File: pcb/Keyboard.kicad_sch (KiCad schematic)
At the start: 63 parts

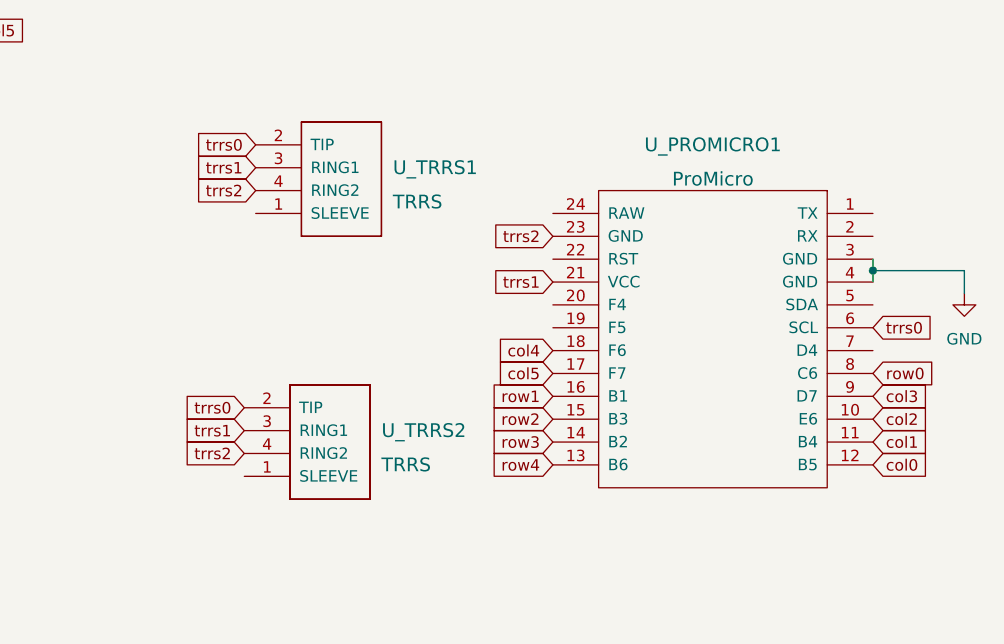
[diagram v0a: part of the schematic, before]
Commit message: wip
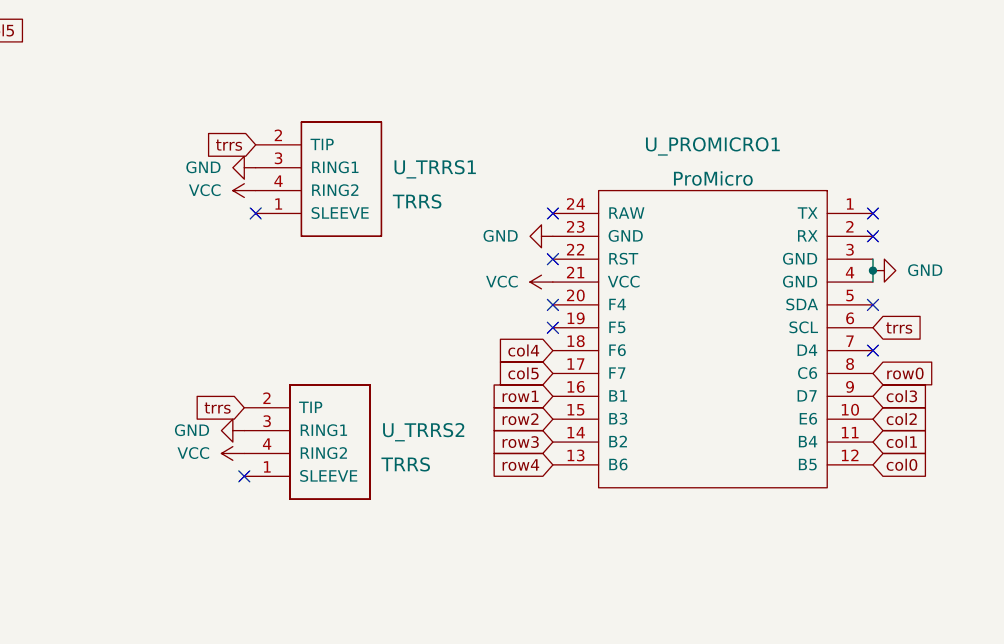
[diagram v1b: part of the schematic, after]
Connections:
- net GND: now also U_PROMICRO1.23 (GND), U_TRRS1.3 (RING1), U_TRRS2.3 (RING1)
- net trrs0 renamed trrs
- removed net trrs1: U_PROMICRO1.21 (VCC), U_TRRS1.3 (RING1), U_TRRS2.3 (RING1)
- net trrs2 renamed VCC
- net VCC: now also U_PROMICRO1.21 (VCC); no longer U_PROMICRO1.23 (GND)
- no-connect marks 0 -> 10

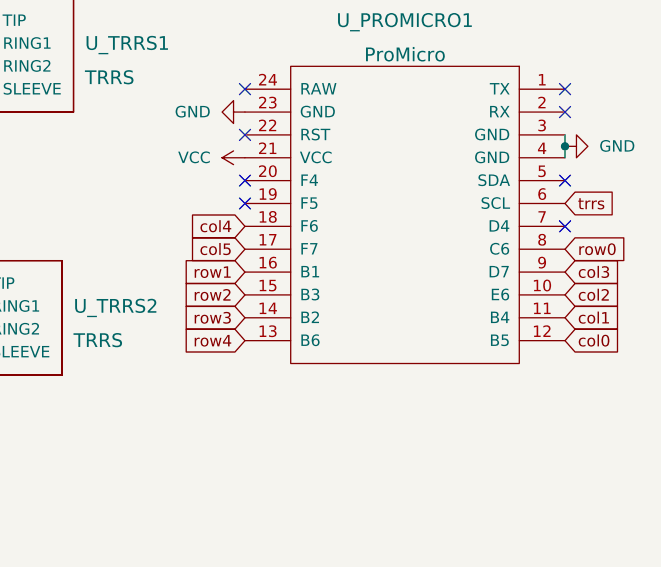
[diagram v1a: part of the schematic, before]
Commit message: wip
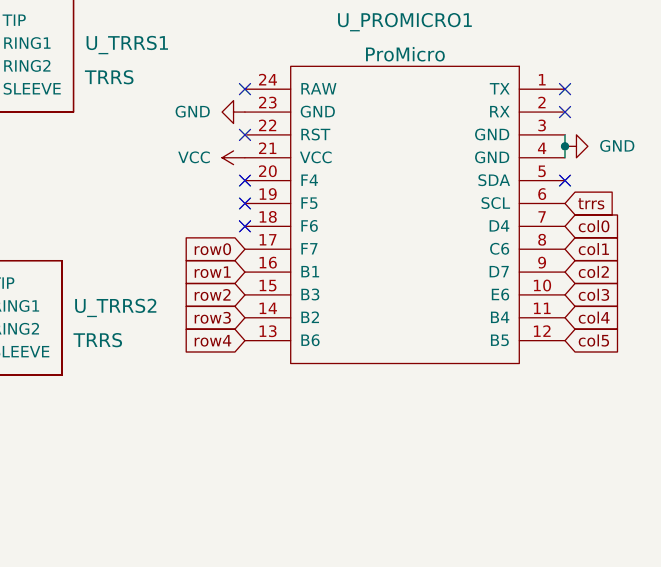
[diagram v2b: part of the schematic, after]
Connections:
- net col0: now also U_PROMICRO1.7 (D4); no longer U_PROMICRO1.12 (B5)
- net col1: now also U_PROMICRO1.8 (C6); no longer U_PROMICRO1.11 (B4)
- net col2: now also U_PROMICRO1.9 (D7); no longer U_PROMICRO1.10 (E6)
- net col3: now also U_PROMICRO1.10 (E6); no longer U_PROMICRO1.9 (D7)
- net col4: now also U_PROMICRO1.11 (B4); no longer U_PROMICRO1.18 (F6)
- net col5: now also U_PROMICRO1.12 (B5); no longer U_PROMICRO1.17 (F7)
- net row0: now also U_PROMICRO1.17 (F7); no longer U_PROMICRO1.8 (C6)
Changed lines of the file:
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@@
   (no_connect (at 262.89 45.72))
   (no_connect (at 262.89 43.18))
-  (no_connect (at 262.89 58.42))
+  (no_connect (at 227.33 58.42))
   (no_connect (at 193.04 72.39))
   (no_connect (at 194.31 43.18))
@@
     (stroke (width 0) (type default) (color 0 0 0 0))
   )
-  (global_label "col5" (shape input) (at 227.33 60.96 180) (fields_autoplaced)
-    (effects (font (size 1.27 1.27)) (justify right))
-    (property "Intersheet References" "${INTERSHEET_REFS}" (id 0) (at 220.8045 60.8806 0)
-      (effects (font (size 1.27 1.27)) (justify right) hide)
-    )
-  )
-  (global_label "col3" (shape input) (at 262.89 63.5 0) (fields_autoplaced)
+  (global_label "col5" (shape input) (at 262.89 71.12 0) (fields_autoplaced)
+    (effects (font (size 1.27 1.27)) (justify left))
+    (property "Intersheet References" "${INTERSHEET_REFS}" (id 0) (at 269.4155 71.0406 0)
+      (effects (font (size 1.27 1.27)) (justify left) hide)
+    )
+  )
+  (global_label "col3" (shape input) (at 262.89 66.04 0) (fields_autoplaced)
+    (effects (font (size 1.27 1.27)) (justify left))
+    (property "Intersheet References" "${INTERSHEET_REFS}" (id 0) (at 269.4155 65.9606 0)
+      (effects (font (size 1.27 1.27)) (justify left) hide)
+    )
+  )
+  (global_label "row4" (shape input) (at 227.33 71.12 180) (fields_autoplaced)
+    (effects (font (size 1.27 1.27)) (justify right))
+    (property "Intersheet References" "${INTERSHEET_REFS}" (id 0) (at 220.4417 71.0406 0)
+      (effects (font (size 1.27 1.27)) (justify right) hide)
+    )
+  )
+  (global_label "trrs" (shape input) (at 194.31 35.56 180) (fields_autoplaced)
+    (effects (font (size 1.27 1.27)) (justify right))
+    (property "Intersheet References" "${INTERSHEET_REFS}" (id 0) (at 188.5707 35.4806 0)
+      (effects (font (size 1.27 1.27)) (justify right) hide)
+    )
+  )
+  (global_label "col4" (shape input) (at 138.43 22.86 0) (fields_autoplaced)
+    (effects (font (size 1.27 1.27)) (justify left))
+    (property "Intersheet References" "${INTERSHEET_REFS}" (id 0) (at 144.9555 22.7806 0)
+      (effects (font (size 1.27 1.27)) (justify left) hide)
+    )
+  )
+  (global_label "row2" (shape input) (at 227.33 66.04 180) (fields_autoplaced)
+    (effects (font (size 1.27 1.27)) (justify right))
+    (property "Intersheet References" "${INTERSHEET_REFS}" (id 0) (at 220.4417 65.9606 0)
+      (effects (font (size 1.27 1.27)) (justify right) hide)
+    )
+  )
+  (global_label "trrs" (shape input) (at 262.89 55.88 0) (fields_autoplaced)
+    (effects (font (size 1.27 1.27)) (justify left))
+    (property "Intersheet References" "${INTERSHEET_REFS}" (id 0) (at 268.6293 55.8006 0)
+      (effects (font (size 1.27 1.27)) (justify left) hide)
+    )
+  )
+  (global_label "col1" (shape input) (at 66.04 22.86 0) (fields_autoplaced)
+    (effects (font (size 1.27 1.27)) (justify left))
+    (property "Intersheet References" "${INTERSHEET_REFS}" (id 0) (at 72.5655 22.7806 0)
+      (effects (font (size 1.27 1.27)) (justify left) hide)
+    )
+  )
+  (global_label "col2" (shape input) (at 262.89 63.5 0) (fields_autoplaced)
     (effects (font (size 1.27 1.27)) (justify left))
     (property "Intersheet References" "${INTERSHEET_REFS}" (id 0) (at 269.4155 63.4206 0)
@@
     )
   )
-  (global_label "row4" (shape input) (at 227.33 71.12 180) (fields_autoplaced)
-    (effects (font (size 1.27 1.27)) (justify right))
-    (property "Intersheet References" "${INTERSHEET_REFS}" (id 0) (at 220.4417 71.0406 0)
-      (effects (font (size 1.27 1.27)) (justify right) hide)
-    )
-  )
-  (global_label "trrs" (shape input) (at 194.31 35.56 180) (fields_autoplaced)
-    (effects (font (size 1.27 1.27)) (justify right))
-    (property "Intersheet References" "${INTERSHEET_REFS}" (id 0) (at 188.5707 35.4806 0)
-      (effects (font (size 1.27 1.27)) (justify right) hide)
-    )
-  )
-  (global_label "col4" (shape input) (at 138.43 22.86 0) (fields_autoplaced)
-    (effects (font (size 1.27 1.27)) (justify left))
-    (property "Intersheet References" "${INTERSHEET_REFS}" (id 0) (at 144.9555 22.7806 0)
-      (effects (font (size 1.27 1.27)) (justify left) hide)
-    )
-  )
-  (global_label "row2" (shape input) (at 227.33 66.04 180) (fields_autoplaced)
-    (effects (font (size 1.27 1.27)) (justify right))
-    (property "Intersheet References" "${INTERSHEET_REFS}" (id 0) (at 220.4417 65.9606 0)
-      (effects (font (size 1.27 1.27)) (justify right) hide)
-    )
-  )
-  (global_label "trrs" (shape input) (at 262.89 55.88 0) (fields_autoplaced)
-    (effects (font (size 1.27 1.27)) (justify left))
-    (property "Intersheet References" "${INTERSHEET_REFS}" (id 0) (at 268.6293 55.8006 0)
-      (effects (font (size 1.27 1.27)) (justify left) hide)
-    )
-  )
-  (global_label "col1" (shape input) (at 66.04 22.86 0) (fields_autoplaced)
-    (effects (font (size 1.27 1.27)) (justify left))
-    (property "Intersheet References" "${INTERSHEET_REFS}" (id 0) (at 72.5655 22.7806 0)
-      (effects (font (size 1.27 1.27)) (justify left) hide)
-    )
-  )
-  (global_label "col2" (shape input) (at 262.89 66.04 0) (fields_autoplaced)
-    (effects (font (size 1.27 1.27)) (justify left))
-    (property "Intersheet References" "${INTERSHEET_REFS}" (id 0) (at 269.4155 65.9606 0)
-      (effects (font (size 1.27 1.27)) (justify left) hide)
-    )
-  )
   (global_label "col3" (shape input) (at 114.3 22.86 0) (fields_autoplaced)
     (effects (font (size 1.27 1.27)) (justify left))
@@
     )
   )
-  (global_label "col4" (shape input) (at 227.33 58.42 180) (fields_autoplaced)
-    (effects (font (size 1.27 1.27)) (justify right))
-    (property "Intersheet References" "${INTERSHEET_REFS}" (id 0) (at 220.8045 58.3406 0)
-      (effects (font (size 1.27 1.27)) (justify right) hide)
+  (global_label "col4" (shape input) (at 262.89 68.58 0) (fields_autoplaced)
+    (effects (font (size 1.27 1.27)) (justify left))
+    (property "Intersheet References" "${INTERSHEET_REFS}" (id 0) (at 269.4155 68.5006 0)
+      (effects (font (size 1.27 1.27)) (justify left) hide)
     )
   )
@@
     )
   )
-  (global_label "row0" (shape input) (at 262.89 60.96 0) (fields_autoplaced)
-    (effects (font (size 1.27 1.27)) (justify left))
-    (property "Intersheet References" "${INTERSHEET_REFS}" (id 0) (at 269.7783 60.8806 0)
-      (effects (font (size 1.27 1.27)) (justify left) hide)
+  (global_label "row0" (shape input) (at 227.33 60.96 180) (fields_autoplaced)
+    (effects (font (size 1.27 1.27)) (justify right))
+    (property "Intersheet References" "${INTERSHEET_REFS}" (id 0) (at 220.4417 60.8806 0)
+      (effects (font (size 1.27 1.27)) (justify right) hide)
     )
   )
@@
     )
   )
-  (global_label "col0" (shape input) (at 262.89 71.12 0) (fields_autoplaced)
-    (effects (font (size 1.27 1.27)) (justify left))
-    (property "Intersheet References" "${INTERSHEET_REFS}" (id 0) (at 269.4155 71.0406 0)
+  (global_label "col0" (shape input) (at 262.89 58.42 0) (fields_autoplaced)
+    (effects (font (size 1.27 1.27)) (justify left))
+    (property "Intersheet References" "${INTERSHEET_REFS}" (id 0) (at 269.4155 58.3406 0)
       (effects (font (size 1.27 1.27)) (justify left) hide)
     )
@@
     )
   )
-  (global_label "col1" (shape input) (at 262.89 68.58 0) (fields_autoplaced)
-    (effects (font (size 1.27 1.27)) (justify left))
-    (property "Intersheet References" "${INTERSHEET_REFS}" (id 0) (at 269.4155 68.5006 0)
-      (effects (font (size 1.27 1.27)) (justify left) hide)
-    )
+  (global_label "col1" (shape input) (at 262.89 60.96 0) (fields_autoplaced)
+    (effects (font (size 1.27 1.27)) (justify left))
+    (property "Intersheet References" "${INTERSHEET_REFS}" (id 0) (at 269.4155 60.8806 0)
+      (effects (font (size 1.27 1.27)) (justify left) hide)
+    )
